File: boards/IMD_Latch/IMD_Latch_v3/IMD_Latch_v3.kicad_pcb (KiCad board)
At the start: 2 copper layers, 37 x 32 mm, 17 parts, among them J1 micromatch_female_RA_8, J2 Ultrafit_2, K1 G5Q-1A4-DC5-5V, Q1 SSM3K333R, U1 CD4043BPWR

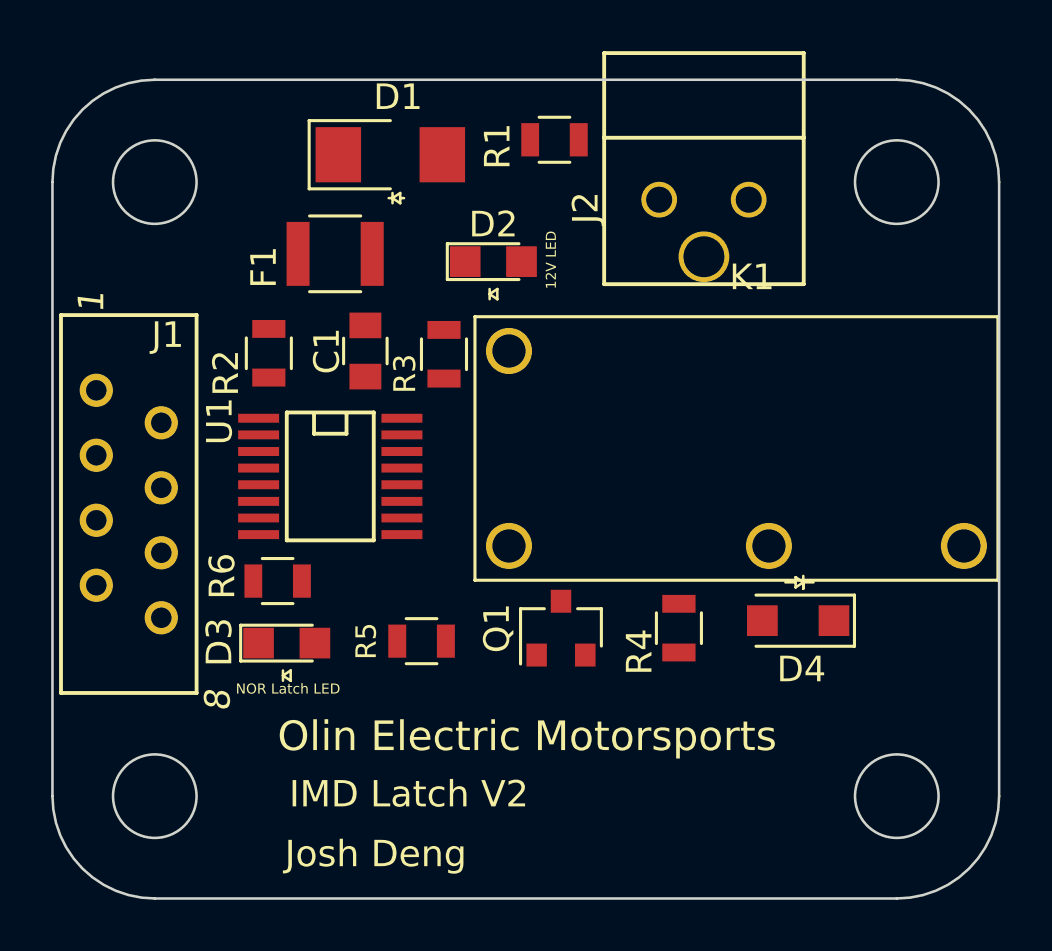
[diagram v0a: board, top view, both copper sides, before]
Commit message: IMD v3 with layout
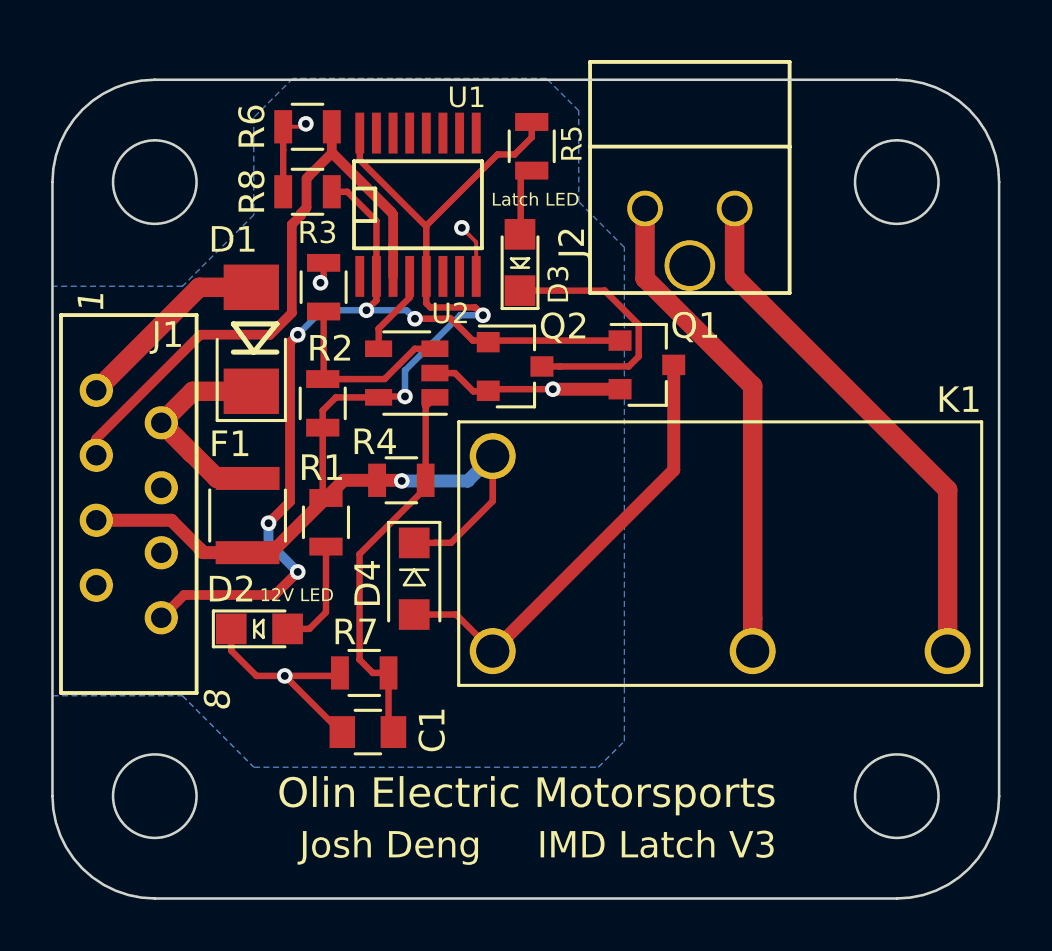
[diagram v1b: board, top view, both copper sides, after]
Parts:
- added G***: LOGO, footprints:Logo_Large, B.Cu at (159.0, 107.2)
- added G***: LOGO, footprints:Olin_O, B.Cu at (156.2, 95.8)
- added Q2: SSM3K333R, footprints:SOT-23F, F.Cu at (158.3, 102.2)
- added R7: R_604k, footprints:R_0805_OEM, F.Cu at (152.4, 114.2)
- added R8: R_604k, footprints:R_0805_OEM, F.Cu at (150.2, 95.4)
- added U2: TLV3701QDBVRG4Q1, footprints:SOT-23-5_OEM, F.Cu at (154.1, 102.5)
- C1: value C_10uF -> C_10uF_16V
- R2: value R_576k -> R_200k
- R3: value R_2.94M -> R_604k
- R4: value R_1M -> R_120k
- moved R5 19.8 mm to (158.9, 93.6), turned to 270 degrees
- moved R6 17.8 mm to (150.2, 92.8), turned to 180 degrees
- moved D3 17.4 mm to (158.5, 98.1), turned to 90 degrees
- moved R1 17.4 mm to (150.9, 108.3), turned to 270 degrees
- moved D2 17.0 mm to (148.3, 112.4)
- moved D4 15.1 mm to (154.3, 110.5), turned to 270 degrees
- moved C1 14.9 mm to (152.5, 116.5), turned to 180 degrees
- moved R4 12.3 mm to (153.8, 106.6), turned to 180 degrees
- moved U1 11.2 mm to (154.5, 95.9), turned to 0 degrees
- moved Q1 10.8 mm to (163.4, 102.1), turned to 0 degrees
- moved F1 10.8 mm to (147.8, 108.0), turned to 270 degrees
- moved D1 9.03 mm to (148.0, 101.1), turned to 90 degrees
- moved R3 5.39 mm to (150.8, 99.1)
- moved K1 4.16 mm to (157.4, 113.3)
- moved R2 2.88 mm to (150.8, 103.6), turned to 90 degrees
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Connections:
- D3 pad 1: GND -> Net-(D3-Pad1)
- J1 pad 8: Net-(J1-Pad8) -> /IMD_Status_Output
- Q1 pad 1: Net-(Q1-Pad1) -> /IMD_Status_Output
- R2 pad 1: Net-(C1-Pad1) -> /12V_Fused
- R2 pad 2: /12V_Fused -> Net-(R2-Pad2)
- R3 pad 1: Net-(C1-Pad1) -> Net-(R2-Pad2)
- R4 pad 1: Net-(Q1-Pad1) -> Net-(C1-Pad1)
- R4 pad 2: GND -> /12V_Fused
- R5 pad 1: Net-(Q1-Pad1) -> /12V_Fused
- U1 pad 1: Net-(U1-Pad1) -> (no net)
- U1 pad 10: Net-(U1-Pad10) -> (no net)
- U1 pad 11: Net-(U1-Pad11) -> (no net)
- U1 pad 12: Net-(U1-Pad12) -> (no net)
- U1 pad 13: Net-(U1-Pad13) -> (no net)
- U1 pad 14: Net-(U1-Pad14) -> (no net)
- U1 pad 15: Net-(U1-Pad15) -> (no net)
- U1 pad 2: Net-(U1-Pad2) -> /IMD_Status_Output
- U1 pad 3: Net-(U1-Pad3) -> Net-(J1-Pad3)
- U1 pad 6: Net-(C1-Pad1) -> (no net)
- U1 pad 7: Net-(J1-Pad3) -> (no net)
- U1 pad 9: Net-(Q1-Pad1) -> (no net)
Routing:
- net /12V_Fused: track 0.00 -> 51.3 mm, vias 0 -> 3
- net /IMD_Status_Output: track 0.00 -> 35.7 mm, vias 0 -> 5
- net Net-(J1-Pad3): track 0.00 -> 30.9 mm
- net GND: track 0.00 -> 30.6 mm, vias 0 -> 5
- net Net-(J2-Pad2): track 0.00 -> 20.7 mm
- net Net-(J2-Pad1): track 0.00 -> 19.0 mm
- net Net-(D4-Pad2): track 0.00 -> 17.8 mm
- net Net-(C1-Pad1): track 0.00 -> 15.2 mm
- net Net-(D3-Pad1): track 0.00 -> 10.4 mm
- net +12V: track 0.00 -> 8.30 mm
- net Net-(R2-Pad2): track 0.00 -> 7.53 mm
- net Net-(D2-Pad2): track 0.00 -> 4.34 mm
- net Net-(U1-Pad4): track 0.00 -> 3.35 mm
- net Net-(D3-Pad2): track 0.00 -> 2.40 mm
- added copper zone on B.Cu, net GND
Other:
- board text added: "IMD Latch V3"
- board text added: "Latch LED"
- board text removed: "IMD Latch V2"
- board text removed: "NOR Latch LED"
